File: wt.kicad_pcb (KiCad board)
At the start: 4 copper layers, 70.9 x 100 mm, 180 parts, among them J1 USB_B, J2 Conn_ARM_JTAG_SWD_10, SW1 SW_Push, SW2 SW_Push, SW3 SW_Push, SW4 SW_Push, SW5 SW_Push, SW6 SW_Push, U1 LM324, U10 LUM-1502-03_3.5mm_mono_vertic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, U11 LUM-1502-03_3.5mm_mono_vertic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, U12 LUM-1502-03_3.5mm_mono_vertic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, U13 LUM-1502-03_3.5mm_mono_vertic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, U14 LUM-1502-03_3.5mm_mono_vertic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, U15 LUM-1502-03_3.5mm_mono_vertic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, U16 power_conn_16, U17 REF191, U18 LM7805_TO220, U19 ZLDO1117G33TA, U2 LM324, U21 LUM-1502-03_3.5mm_mono_vertic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, U22 LUM-1502-03_3.5mm_mono_vertic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, U23 LUM-1502-03_3.5mm_mono_vertic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, U24 LUM-1502-03_3.5mm_mono_vertic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, U3 LM324, U4 STM32F407VGTx, U5 TL074, U6 TL074, U7 TLC7528, U8 LUM-1502-03_3.5mm_mono_vertic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, U9 LUM-1502-03_3.5mm_mono_vertic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, Y1 Crystal_8Mhz

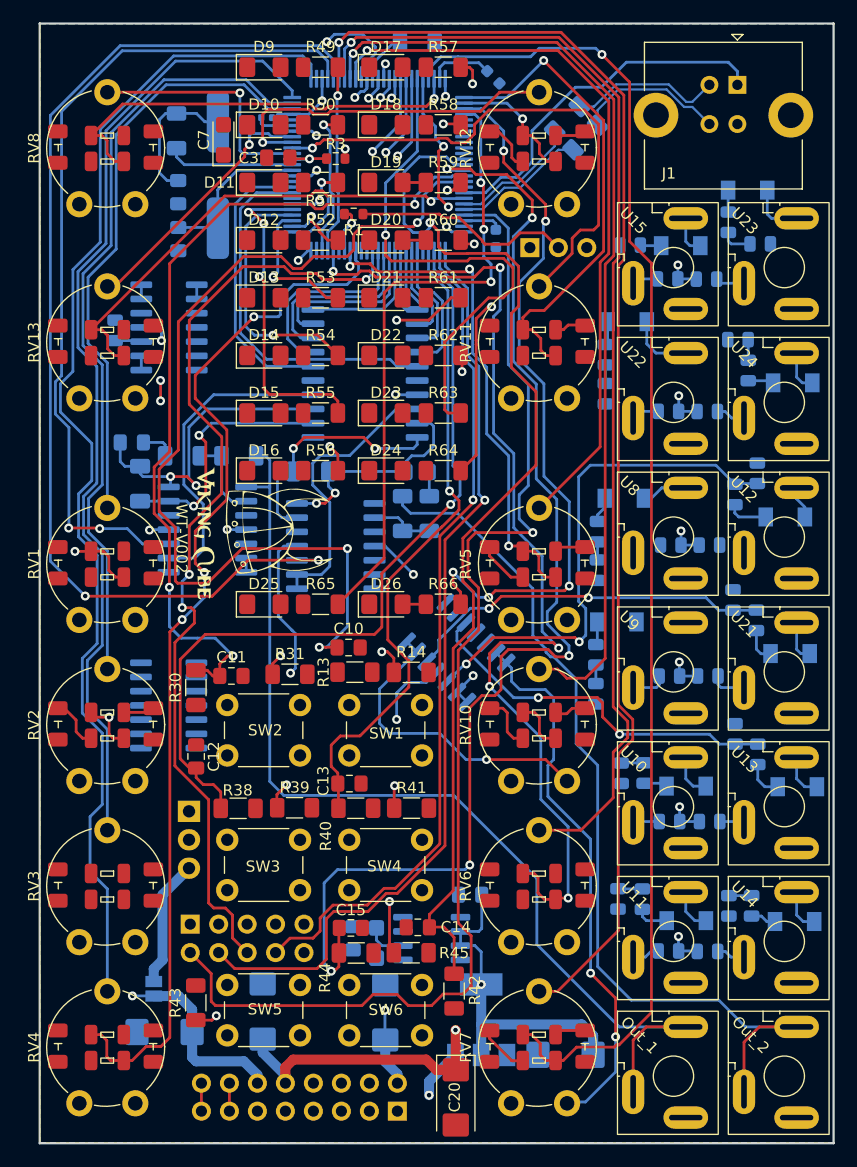
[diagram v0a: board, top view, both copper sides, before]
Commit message: Moved around a lot, I think we close to GND phase
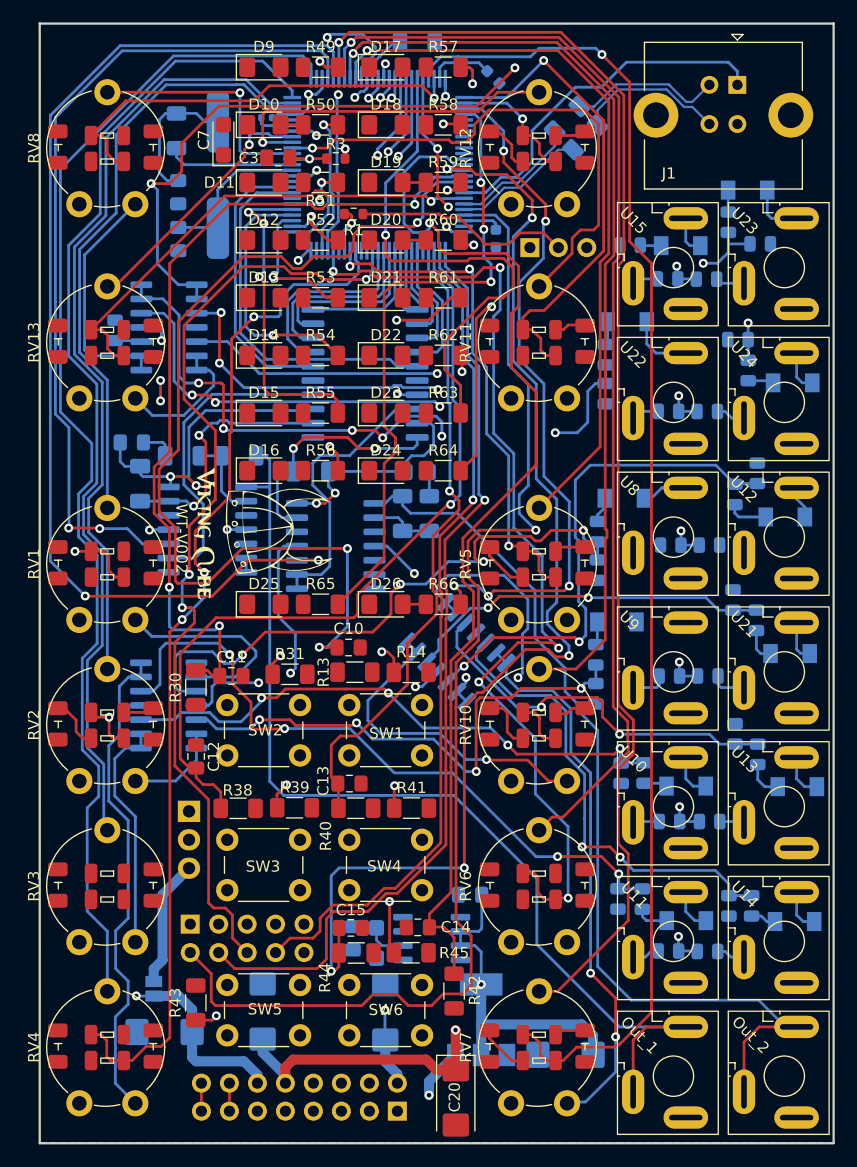
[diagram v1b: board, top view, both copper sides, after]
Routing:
- net Net-(RV12-Pad1): track 1.27 -> 65.6 mm, vias 0 -> 2
- net Net-(R79-Pad2): track 1.85 -> 65.4 mm, vias 0 -> 2
- net Net-(R76-Pad2): track 2.82 -> 63.5 mm, vias 0 -> 4
- net Net-(R25-Pad2): track 2.19 -> 61.2 mm, vias 0 -> 4
- net Net-(RV11-Pad1): track 1.27 -> 56.5 mm, vias 0 -> 5
- net Net-(R16-Pad2): track 1.62 -> 54.3 mm, vias 0 -> 4
- net Net-(R73-Pad2): track 1.66 -> 54.0 mm, vias 0 -> 4
- net Net-(R22-Pad2): track 2.06 -> 50.8 mm, vias 0 -> 4
- net Net-(RV6-Pad1): track 0.00 -> 48.6 mm, vias 0 -> 1
- net Net-(R19-Pad2): track 1.66 -> 47.2 mm, vias 0 -> 4
- net Net-(RV4-Pad1): track 0.00 -> 44.0 mm
- net Net-(R36-Pad2): track 2.03 -> 42.3 mm, vias 0 -> 2
- net +3V3: track 351.4 -> 374.7 mm, vias 17 -> 18
- net Net-(RV3-Pad1): track 0.00 -> 21.1 mm
- net Net-(RV8-Pad1): track 1.27 -> 21.5 mm
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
